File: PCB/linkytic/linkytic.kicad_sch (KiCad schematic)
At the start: 14 parts, among them U1 M5333B, U2 cc2530

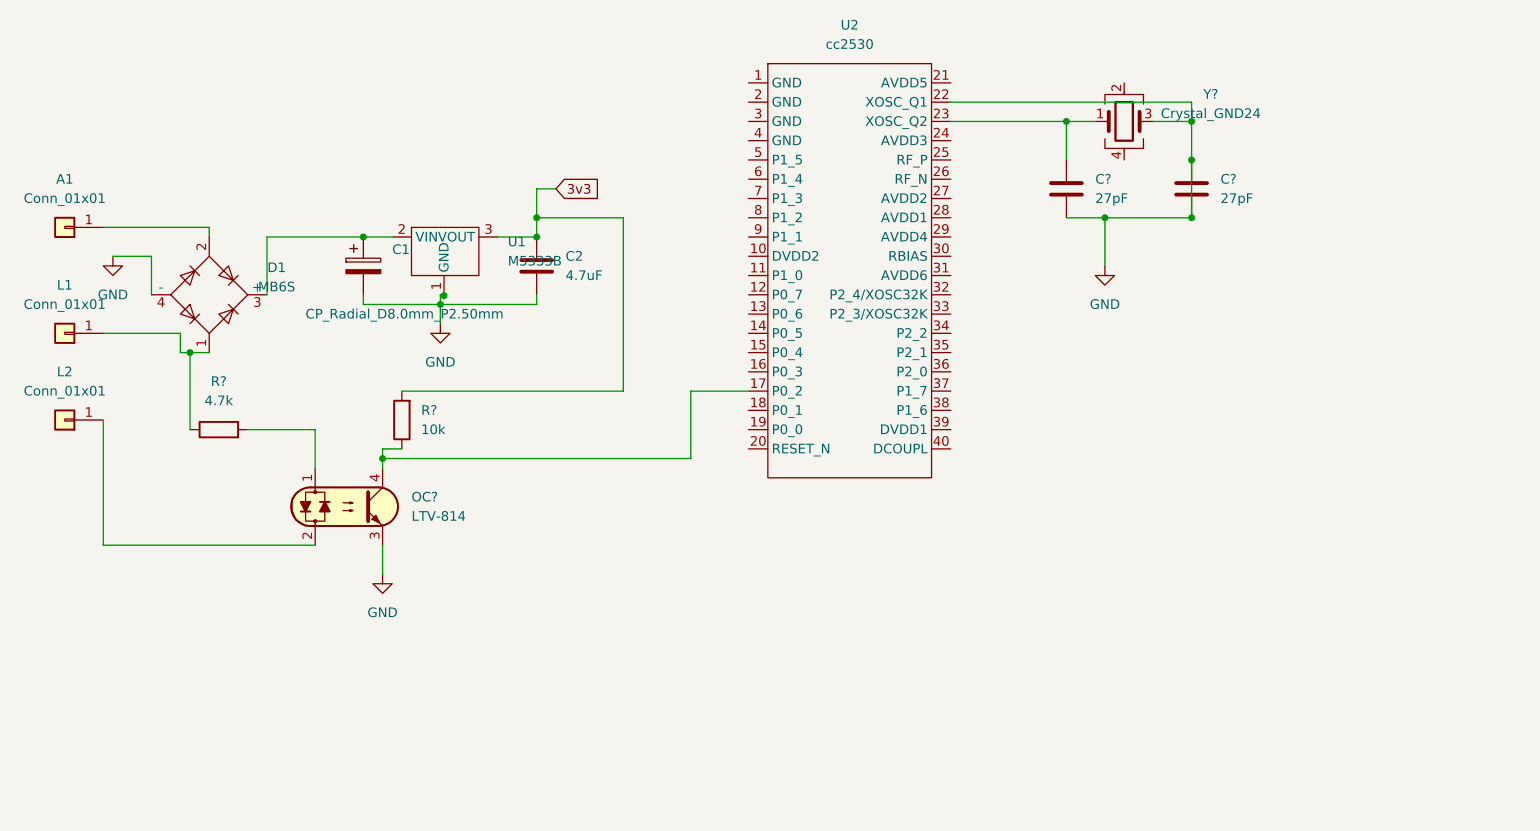
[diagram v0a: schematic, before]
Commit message: v0
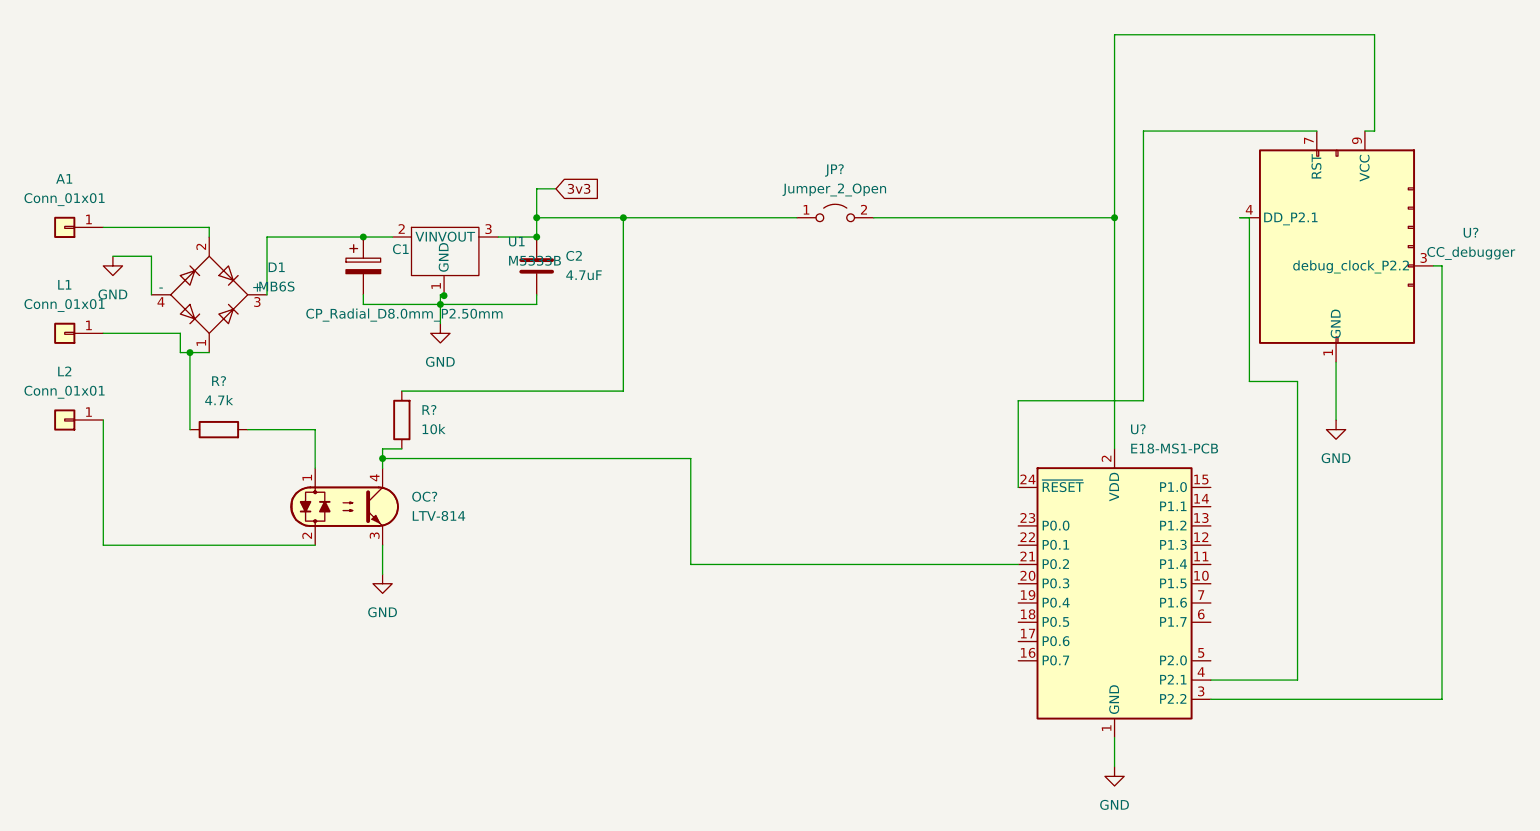
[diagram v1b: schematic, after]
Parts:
- removed C? (x2): 27pF, Capacitor_SMD:C_0603_1608Metric, symbol Device:C
- removed U2: cc2530, Package_DFN_QFN:HVQFN-40-1EP_6x6mm_P0.5mm_EP4.1x4.1mm, symbol cc2530:cc2530
- removed Y?: Crystal_GND24, symbol Device:Crystal_GND24
- added JP?: Jumper_2_Open, symbol Jumper:Jumper_2_Open
- added U?: CC_debugger, Connector_IDC:IDC-Header_2x05_P2.54mm_Vertical, symbol cc_debugger:CC_debugger
- added U?: E18-MS1-PCB, RF_Module:E18-MS1-PCB, symbol RF_Module:E18-MS1-PCB
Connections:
- net 3v3: now also JP?.1 (A)
- net GND: now also U?.1 (GND), U?.1 (GND)
- net at OC?.4, R?.1: now also U?.21 (P0.2)
- new net: JP?.2 (B), U?.2 (VDD), U?.9 (VCC)
- new net: U?.3 (P2.2), U?.3 (debug_clock_P2.2)
- new net: U?.4 (DD_P2.1), U?.4 (P2.1)
- new net: U?.24 (~{RESET}), U?.7 (RST)
